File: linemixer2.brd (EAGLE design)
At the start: 95.2 x 59.7 mm, 82 parts, among them IC1 OPA2134P, IC2 OPA2134P, IC3 OPA2134P, IC4 OPA2134P, IC5 OPA2134P, J1 POWER_JACK

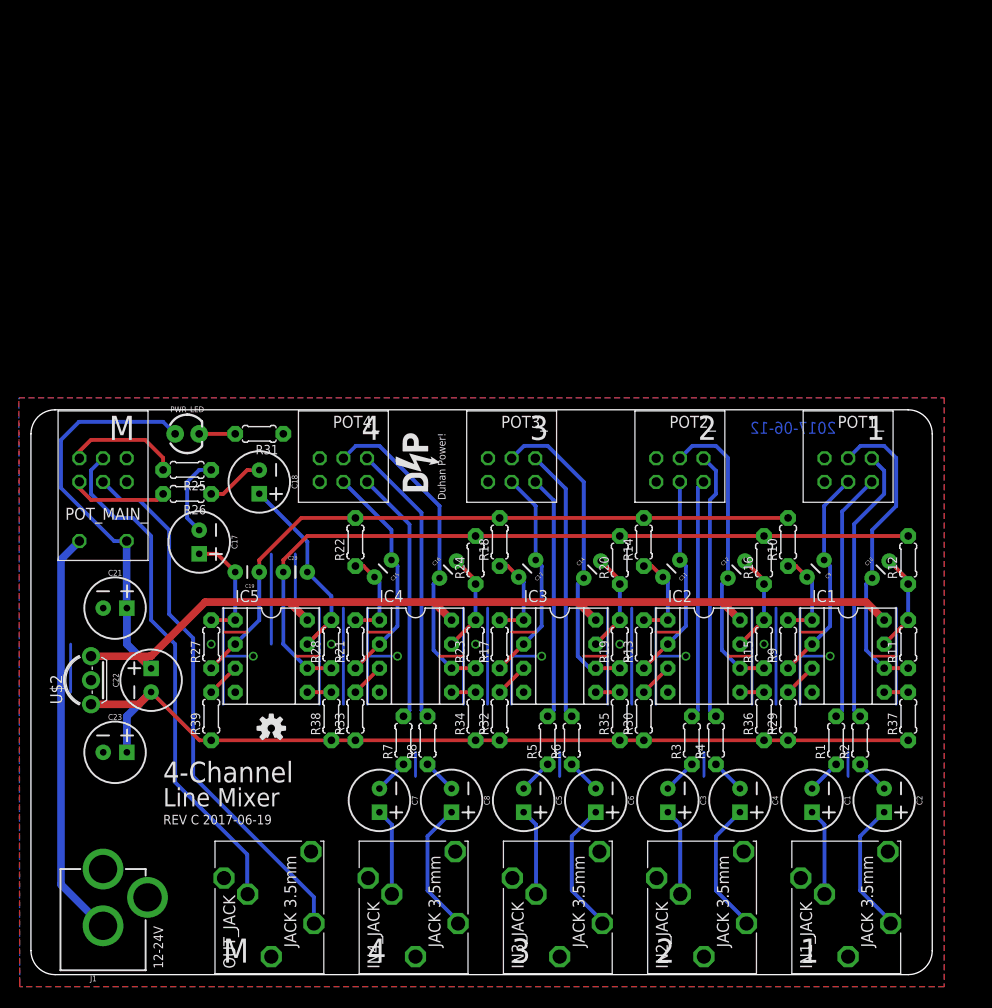
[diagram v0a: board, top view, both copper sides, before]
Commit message: rev D
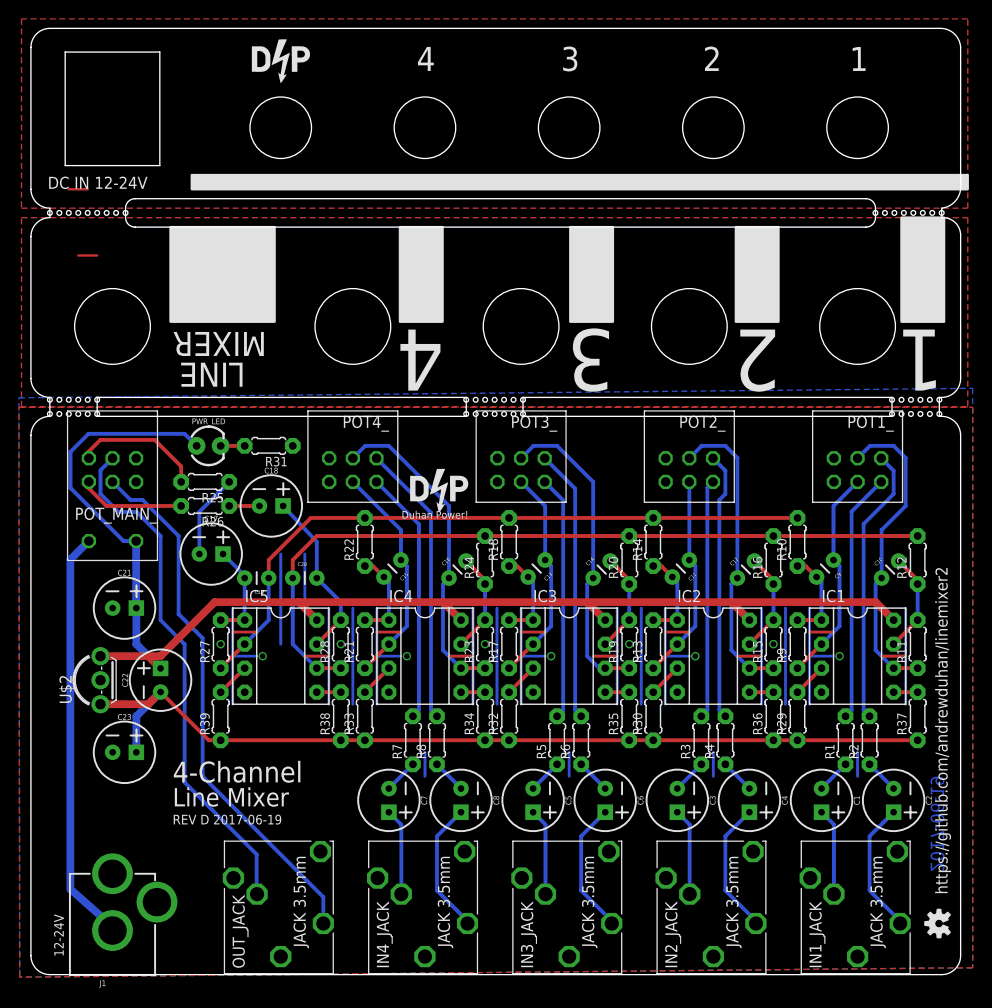
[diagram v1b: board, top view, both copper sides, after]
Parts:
- added U$3: DP_LOGO, myparts:DP_LOGO
- moved LOGO1 73.5 mm to (96.0, 5.40), turned to 90 degrees
- moved U$1 3.51 mm to (43.0, 51.4), turned to 0 degrees
- moved C18 2.84 mm to (25.4, 49.5), turned to 0 degrees
- moved PWR_LED 2.60 mm to (18.8, 55.9)
- moved R25 2.29 mm to (18.4, 52.1)
- moved R26 2.29 mm to (18.4, 49.5)
- moved C17 1.80 mm to (19.1, 44.5), turned to 0 degrees
- moved R31 1.62 mm to (25.1, 55.9)
- moved C19 1.18 mm to (25.1, 41.9)
- moved C20 1.18 mm to (27.7, 41.9)
- moved J1 1.12 mm to (8.62, -3.04)
- moved C1 1.00 mm to (83.5, 18.4)
- moved C10 1.00 mm to (89.9, 41.9)
- moved C11 1.00 mm to (69.6, 43.8)
- moved C12 1.00 mm to (74.7, 41.9)
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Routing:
- net GND: track 210.8 -> 205.7 mm
- net N$36: track 6.12 -> 3.20 mm
- net G4: track 0.00 -> 2.00 mm
- net G3: track 0.00 -> 2.00 mm
- net N$23: track 20.1 -> 18.1 mm
- net N$22: track 12.2 -> 10.5 mm
- net N$37: track 12.2 -> 13.8 mm
- net N$41: track 3.81 -> 2.54 mm
- net N$38: track 10.3 -> 11.2 mm
- net N$42: track 43.4 -> 43.9 mm
- added copper zone on layer 1, net G3
- added copper zone on layer 1, net G4
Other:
- board size 95.2 x 59.7 mm -> 98.3 x 100 mm
- board text added: "2017-06-19"
- board text added: "DC IN 12-24V"
- board text added: "LINE"
- board text added: "MIXER"
- board text added: "REV D 2017-06-19"
- board text added: "https://github.com/andrewduhan/linemixer2"
- board text removed: "2017-06-12"
- board text removed: "M"
- board text removed: "REV C 2017-06-19"
